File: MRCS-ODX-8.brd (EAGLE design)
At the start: 150 x 69 mm, 19 parts, among them CON1 INPUT (3.96), CON4 CONNECTOR-M035MM-LOCK

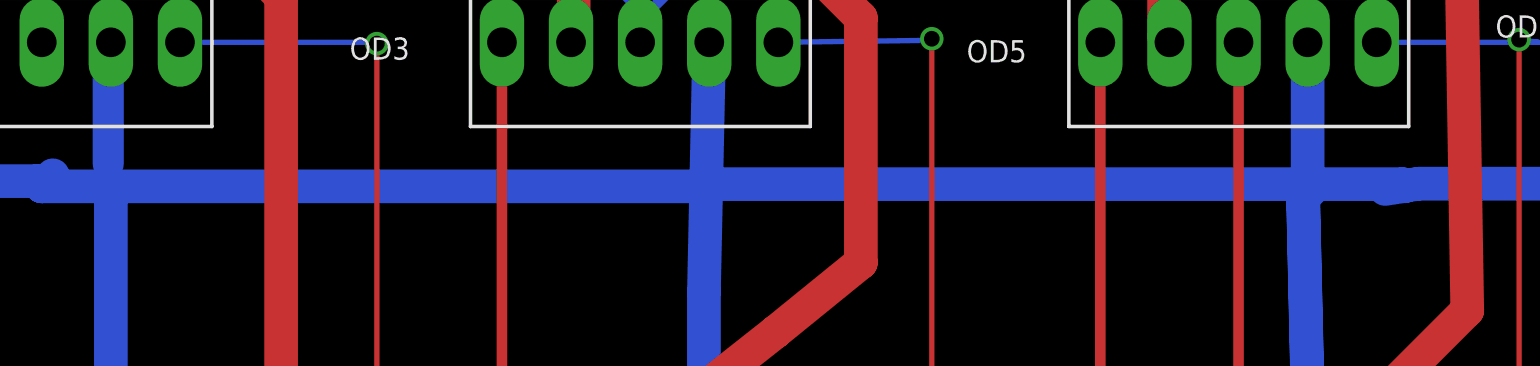
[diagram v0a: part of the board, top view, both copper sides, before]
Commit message: minor changes and new gerbers
revised gerbers
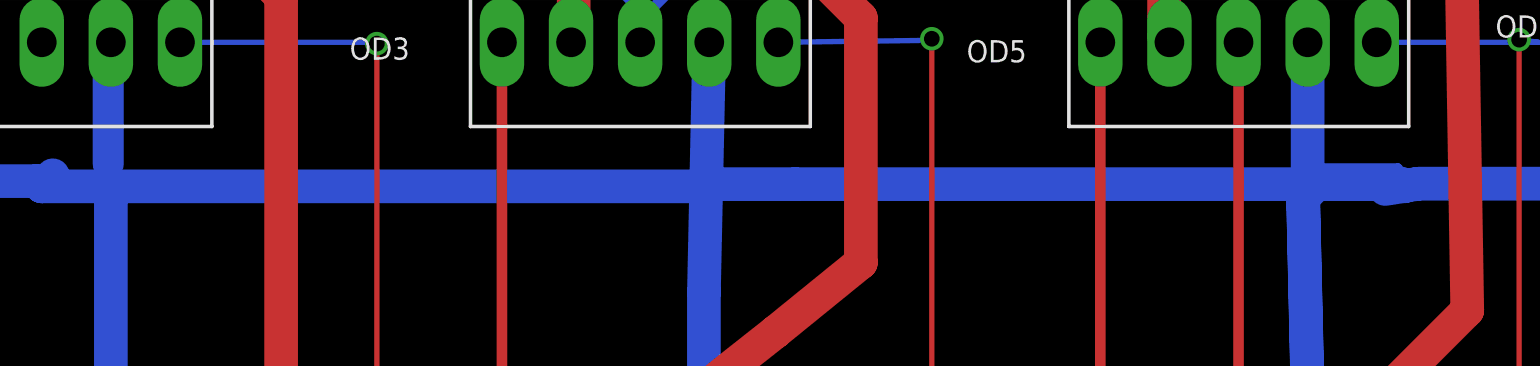
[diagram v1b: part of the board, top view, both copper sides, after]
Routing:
- net TRACK_POWER: track 310.9 -> 354.3 mm
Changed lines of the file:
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@@
 <setting verticaltext="up"/>
 </settings>
-<grid distance="25" unitdist="mil" unit="mil" style="dots" multiple="2" display="yes" altdistance="25" altunitdist="mil" altunit="mil"/>
+<grid distance="50" unitdist="mil" unit="mil" style="dots" multiple="2" display="yes" altdistance="25" altunitdist="mil" altunit="mil"/>
 <layers>
 <layer number="1" name="Top" color="4" fill="1" visible="yes" active="yes"/>
@@
 <wire x1="68.554090625" y1="40.640553125" x2="68.4252" y2="34.5924" width="1.9304" layer="16"/>
 <wire x1="103.02" y1="28.344" x2="102.743" y2="40.767" width="1.9304" layer="16"/>
-<wire x1="102.743" y1="40.767" x2="68.453" y2="40.767" width="1.9304" layer="16"/>
+<wire x1="102.743" y1="40.767" x2="73.66" y2="40.767" width="1.9304" layer="16"/>
+<wire x1="73.66" y1="40.767" x2="68.453" y2="40.767" width="1.9304" layer="16"/>
 <wire x1="103.0454" y1="15.875" x2="103.0454" y2="27.7138" width="1.9304" layer="16"/>
 <wire x1="103.0454" y1="27.7138" x2="102.761053125" y2="39.987765625" width="1.9304" layer="16"/>
@@
 <wire x1="68.4252" y1="34.5924" x2="68.4252" y2="16.8148" width="1.9304" layer="16"/>
 <wire x1="68.4252" y1="16.8148" x2="68.73" y2="16.51" width="1.9304" layer="16"/>
-<wire x1="109.37" y1="40.7924" x2="107.465" y2="40.49" width="1.9304" layer="16"/>
+<wire x1="109.37" y1="40.7924" x2="109.200090625" y2="40.765428125" width="1.9304" layer="16"/>
+<wire x1="109.200090625" y1="40.765428125" x2="107.465" y2="40.49" width="1.9304" layer="16"/>
 <wire x1="103.4132875" y1="40.64" x2="102.761053125" y2="39.987765625" width="1.9304" layer="16"/>
 <wire x1="103.02" y1="48.895" x2="103.02" y2="41.76" width="1.9304" layer="16"/>
@@
 <wire x1="132.865" y1="50.165" x2="132.865" y2="40.0074" width="1.9304" layer="16"/>
 <wire x1="132.865" y1="40.0074" x2="135.255" y2="40.7924" width="1.9304" layer="16"/>
-<wire x1="108.585" y1="40.64" x2="109.37" y2="40.7924" width="0" layer="19" extent="16-16"/>
+<wire x1="34.29" y1="41.91" x2="34.29" y2="40.64" width="0.4064" layer="16"/>
+<wire x1="103.02" y1="41.76" x2="108.20551875" y2="41.76" width="0.4064" layer="16"/>
+<wire x1="108.20551875" y1="41.76" x2="109.200090625" y2="40.765428125" width="0.4064" layer="16"/>
+<wire x1="109.200090625" y1="40.765428125" x2="73.661571875" y2="40.765428125" width="0.4064" layer="16"/>
+<wire x1="73.661571875" y1="40.765428125" x2="73.66" y2="40.767" width="0.4064" layer="16"/>
 <wire x1="68.554090625" y1="40.640553125" x2="68.453" y2="40.767" width="0" layer="19" extent="16-16"/>
 <wire x1="7.62" y1="40.64" x2="7.62" y2="40.94" width="0" layer="19" extent="16-16"/>
-<wire x1="103.02" y1="41.76" x2="102.743" y2="40.767" width="0" layer="19" extent="16-16"/>
-<wire x1="34.29" y1="41.91" x2="34.29" y2="40.64" width="0" layer="19" extent="16-16"/>
 </signal>
 <signal name="N$1">
